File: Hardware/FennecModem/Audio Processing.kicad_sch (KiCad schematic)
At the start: 14 parts, among them U1 MCP6022

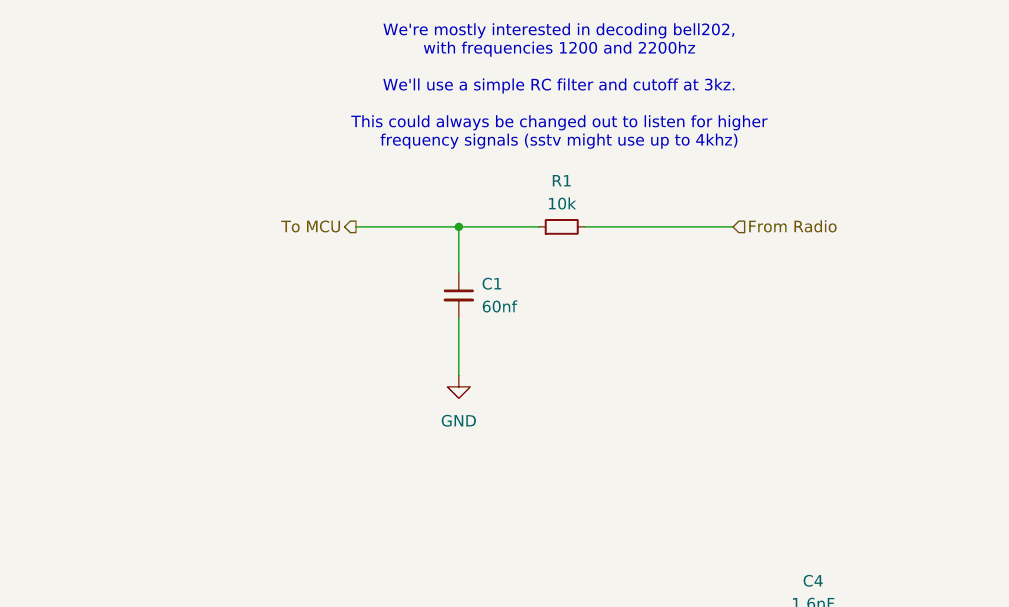
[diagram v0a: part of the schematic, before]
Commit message: Route!
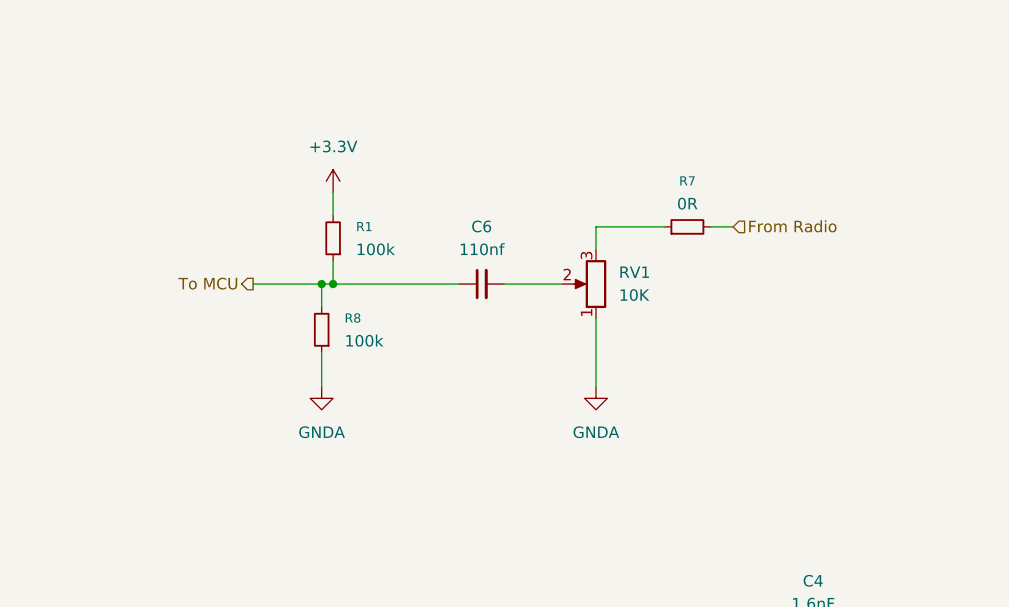
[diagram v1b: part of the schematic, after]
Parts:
- removed C1: 60nf, Capacitor_THT:CP_Radial_D4.0mm_P2.00mm, symbol Device:C_Small
- added C6: 110nf, Capacitor_SMD:C_0805_2012Metric, symbol Device:C_Small
- added R7: 0R, Resistor_SMD:R_0805_2012Metric, symbol Device:R_Small
- added R8: 100k, Resistor_SMD:R_0805_2012Metric, symbol Device:R_Small
- added RV1: 10K, Potentiometer_SMD:Potentiometer_Bourns_TC33X_Vertical, symbol Device:R_Potentiometer
- R1: value 10k -> 100k; footprint Resistor_THT:R_Axial_DIN0207_L6.3mm_D2.5mm_P10.16mm_Horizontal -> Resistor_SMD:R_0805_2012Metric
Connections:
- net +3.3V: now also R1.2
- net From Radio: now also R7.2; no longer R1.2
- net To MCU: now also C6.1, R8.2
- new net: R7.1, RV1.3
- new net: C6.2, RV1.2
- new net GNDA: R8.1, RV1.1
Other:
- note removed: "We're mostly interested in decoding bell202, with frequencies 1200 and 2200hz We'll use a simple RC filter and cutoff at 3kz. This could always be changed out to listen for higher frequency signals (sstv might use up to 4khz)"
